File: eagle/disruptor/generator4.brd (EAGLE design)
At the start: 126.5 x 120.7 mm, 36 parts, among them IC1 NE555, IC2 74ALS04N, IC3 IR2110, IC4 7805TV, J1 PIN2F061.100, J2 PIN2F061.100, J3 PIN2F061.100, J4 PIN2F061.100, J5 PIN2F061.100, J6 PIN2F061.100, Q1 STP11NM60, Q2 STP11NM60

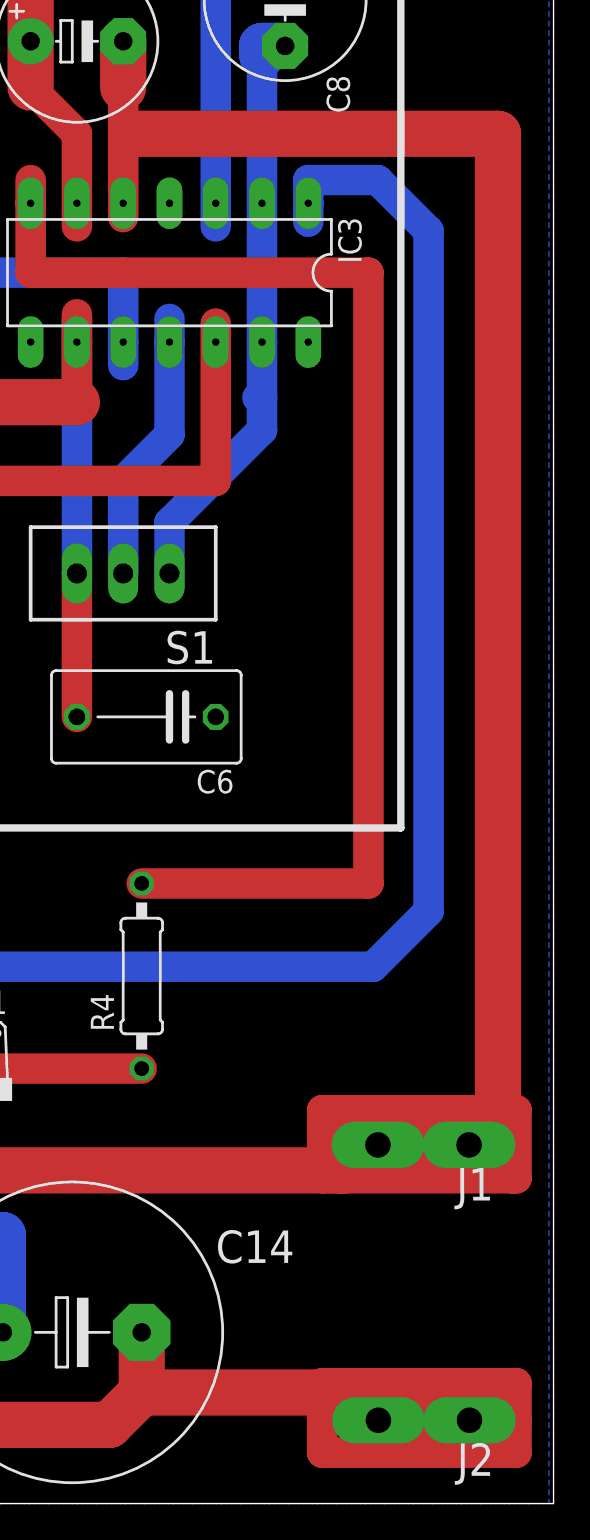
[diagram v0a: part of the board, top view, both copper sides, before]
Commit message: final board
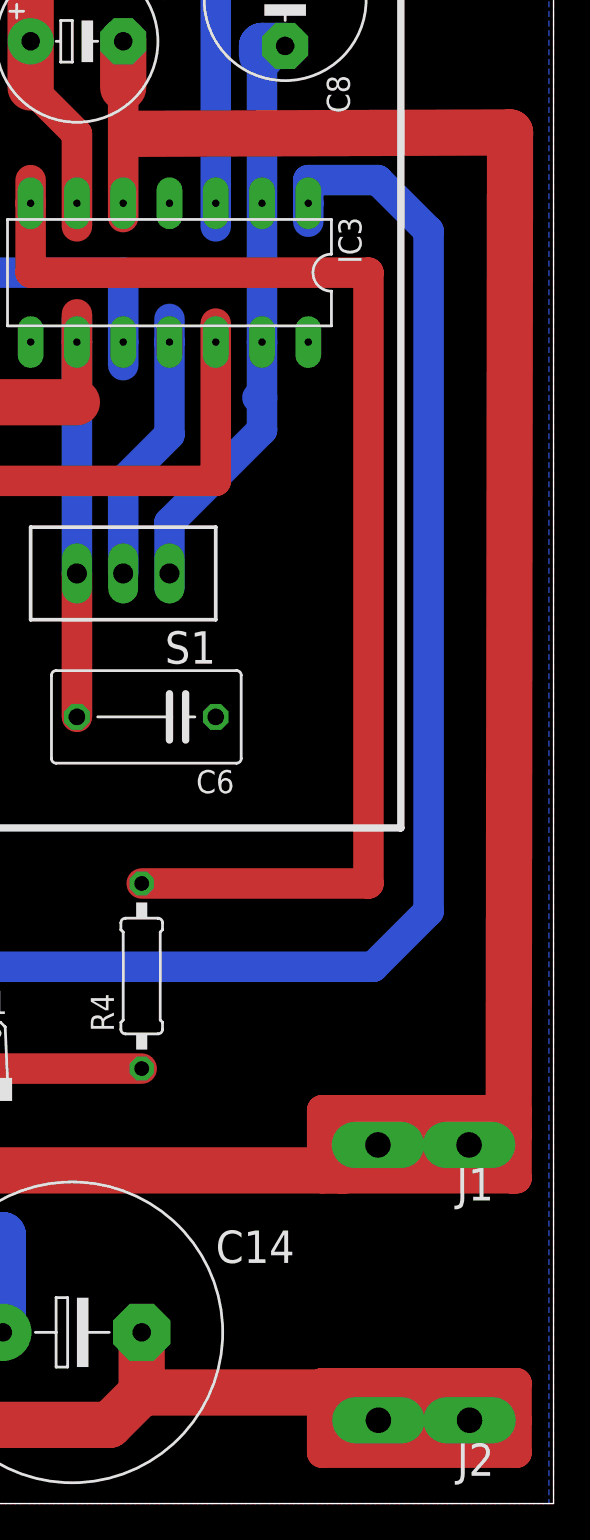
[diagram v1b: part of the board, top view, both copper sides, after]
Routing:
- net N$8: track 95.7 -> 99.3 mm
- net TRANS: track 221.4 -> 223.1 mm
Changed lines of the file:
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@@
 <wire x1="52.578" y1="80.01" x2="52.578" y2="77.47" width="2.54" layer="1"/>
 <wire x1="52.578" y1="70.358" x2="52.578" y2="77.47" width="1.6764" layer="1"/>
-<wire x1="73.152" y1="74.93" x2="53.086" y2="74.93" width="2.54" layer="1"/>
+<wire x1="73.8124" y1="75.0062" x2="53.086" y2="74.93" width="2.54" layer="1"/>
 <wire x1="71.5626" y1="19.431" x2="73.152" y2="19.812" width="2.54" layer="1"/>
-<wire x1="73.152" y1="19.812" x2="73.152" y2="20.066" width="2.54" layer="1"/>
-<wire x1="73.152" y1="20.066" x2="73.152" y2="74.93" width="2.54" layer="1"/>
+<wire x1="73.152" y1="19.812" x2="73.7362" y2="19.939" width="2.54" layer="1"/>
+<wire x1="73.7362" y1="19.939" x2="73.8124" y2="75.0062" width="2.54" layer="1"/>
 <wire x1="38.608" y1="24.384" x2="38.608" y2="28.448" width="1.6764" layer="1"/>
 <wire x1="38.608" y1="28.448" x2="33.528" y2="33.274" width="1.6764" layer="1"/>
@@
 <wire x1="64.516" y1="17.6022" x2="64.516" y2="20.32" width="1.6764" layer="1"/>
 <wire x1="64.516" y1="20.32" x2="72.898" y2="20.32" width="1.6764" layer="1"/>
-<wire x1="72.898" y1="20.32" x2="73.152" y2="20.066" width="1.6764" layer="1"/>
+<wire x1="72.898" y1="20.32" x2="73.7362" y2="19.939" width="1.6764" layer="1"/>
 <wire x1="66.5626" y1="19.431" x2="66.802" y2="19.558" width="1.6764" layer="1"/>
 <wire x1="66.802" y1="19.558" x2="68.072" y2="18.288" width="1.6764" layer="1"/>
@@
 <wire x1="65.024" y1="5.842" x2="66.588" y2="4.318" width="2.54" layer="1"/>
 <wire x1="66.588" y1="4.318" x2="72.898" y2="4.318" width="2.54" layer="1"/>
-<wire x1="66.588" y1="4.318" x2="74.168" y2="4.318" width="1.6764" layer="1"/>
+<wire x1="72.898" y1="4.318" x2="74.168" y2="4.318" width="1.6764" layer="1"/>
 <wire x1="74.168" y1="4.318" x2="74.168" y2="6.35" width="1.6764" layer="1"/>
 <wire x1="74.168" y1="6.35" x2="72.39" y2="6.35" width="1.6764" layer="1"/>
@@
 <wire x1="63.5" y1="6.35" x2="72.39" y2="6.35" width="1.6764" layer="1"/>
 <wire x1="72.39" y1="6.35" x2="72.898" y2="5.842" width="1.6764" layer="1"/>
-<wire x1="72.898" y1="4.318" x2="71.588" y2="4.318" width="0" layer="19" extent="1-1"/>
 <wire x1="24.638" y1="8.89" x2="24.638" y2="9.398" width="0" layer="19" extent="1-1"/>
+<wire x1="72.898" y1="4.318" x2="64.7446" y2="4.318" width="1.6764" layer="1"/>
+<wire x1="64.7446" y1="4.318" x2="64.7446" y2="3.8354" width="1.6764" layer="1"/>
+<wire x1="64.7446" y1="3.8354" x2="65.6336" y2="3.8354" width="1.6764" layer="1"/>
+<wire x1="65.6336" y1="3.8354" x2="65.6336" y2="3.5052" width="1.6764" layer="1"/>
+<wire x1="65.6336" y1="3.5052" x2="71.588" y2="4.318" width="0" layer="19" extent="1-16"/>
 </signal>
 </signals>
